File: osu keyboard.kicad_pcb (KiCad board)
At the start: 2 copper layers, 79.4 x 73.8 mm, 25 parts, among them SW1 SW_Push, U1 ATmega32U4-A, U2 PRTR5V0U2X, Y1 16MHz

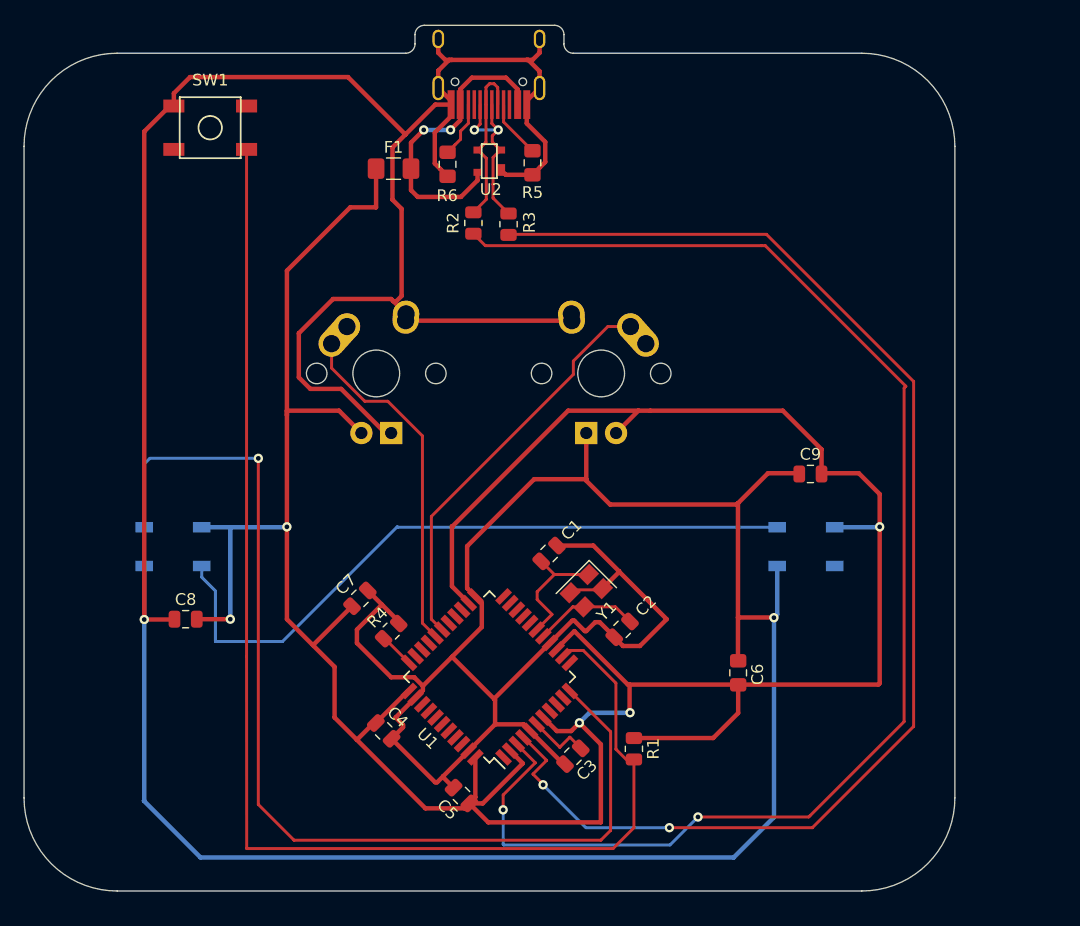
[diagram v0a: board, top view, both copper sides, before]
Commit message: using rp2040
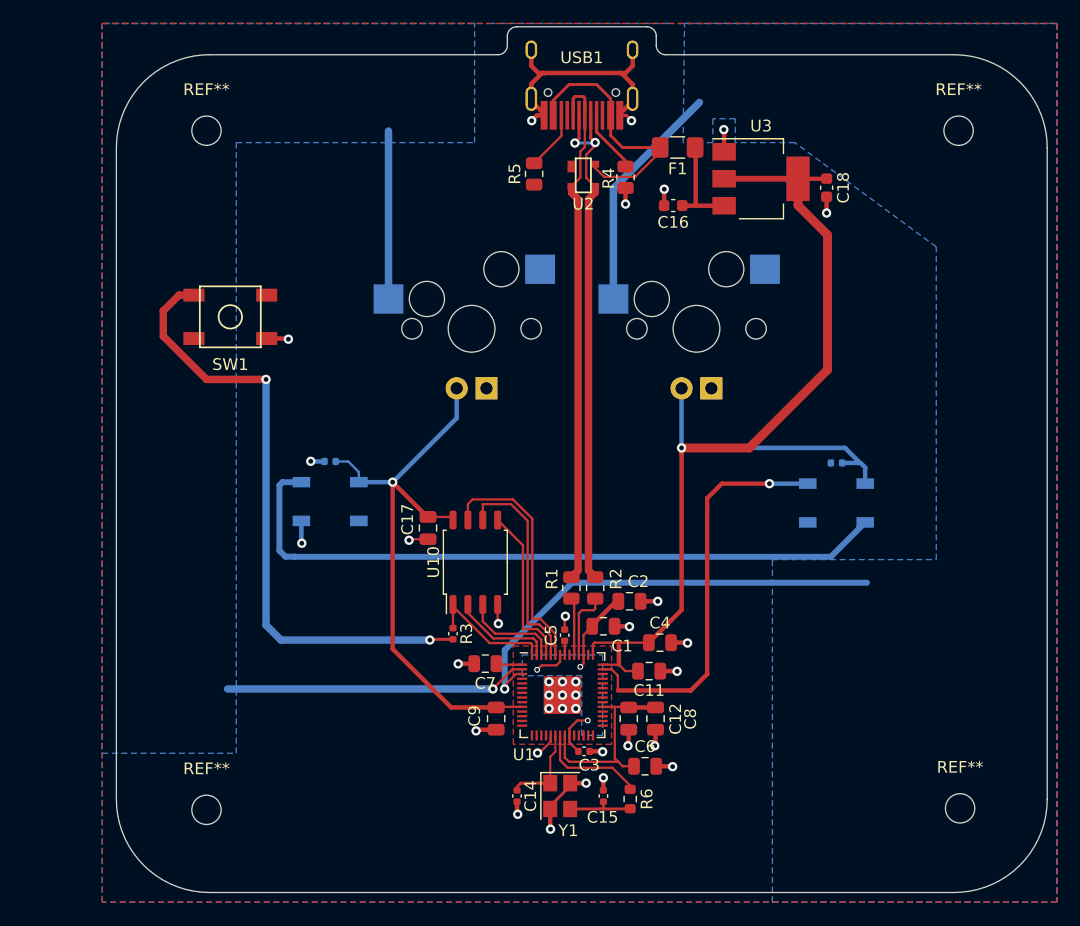
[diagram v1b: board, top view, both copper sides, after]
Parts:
- added C10: 100nF, Capacitor_SMD:C_0402_1005Metric, B.Cu at (156.6, 98.4)
- added C11: 100nF, Capacitor_SMD:C_0805_2012Metric, F.Cu at (140.6, 116.2)
- added C12: 100nF, Capacitor_SMD:C_0805_2012Metric, F.Cu at (138.9, 120.2)
- added C13: 100nF, Capacitor_SMD:C_0402_1005Metric, B.Cu at (113.4, 98.3)
- added C14: 14pF, Capacitor_SMD:C_0402_1005Metric, F.Cu at (129.3, 126.8)
- added C15: 14pF, Capacitor_SMD:C_0402_1005Metric, F.Cu at (136.7, 126.8)
- added C16: 22uF, Capacitor_SMD:C_0603_1608Metric, F.Cu at (142.7, 76.5)
- added C17: 100nF, Capacitor_SMD:C_0805_2012Metric, F.Cu at (121.8, 104.0)
- added C18: 22uF, Capacitor_SMD:C_0603_1608Metric, F.Cu at (155.7, 75.0)
- added REF**: MountingHole_2.5mm, MountingHole:MountingHole_2.5mm, F.Cu at (167.1, 127.9)
- added REF**: MountingHole_2.5mm, MountingHole:MountingHole_2.5mm, F.Cu at (167.0, 70.1)
- added REF**: MountingHole_2.5mm, MountingHole:MountingHole_2.5mm, F.Cu at (102.9, 70.1)
- added REF**: MountingHole_2.5mm, MountingHole:MountingHole_2.5mm, F.Cu at (102.9, 128.0)
- added U10: W25Q128JVS, Package_SO:SOIC-8_5.23x5.23mm_P1.27mm, F.Cu at (125.8, 106.9)
- added U3: AMS1117-3.3, Package_TO_SOT_SMD:SOT-223-3_TabPin2, F.Cu at (150.2, 74.2)
- C1, C2: value 22pF -> 100nF
- C3: footprint Capacitor_SMD:C_0805_2012Metric -> Capacitor_SMD:C_0402_1005Metric
- C4, C8, C9: value 0.1uF -> 100nF
- C5: value 0.1uF -> 1uF; footprint Capacitor_SMD:C_0805_2012Metric -> Capacitor_SMD:C_0402_1005Metric
- C6: value 10uF -> 100nF; footprint Capacitor_SMD:C_0805_2012Metric_Pad1.15x1.40mm_HandSolder -> Capacitor_SMD:C_0805_2012Metric
- C7: value 10uf -> 100nF
- F1: value 500mA -> Polyfuse_Small
- MX0: footprint MX_Alps_Hybrid:MX-1U -> MX_Only:MXOnly-1U-Hotswap-LED
- MX1: footprint MX_Alps_Hybrid:MX-1U -> MX_Only:MXOnly-1U-Hotswap-LED; moved to F.Cu
- R1: value 10k -> 27
- R2: value 22 -> 27
- R3: value 22 -> 1k; footprint Resistor_SMD:R_0805_2012Metric -> Capacitor_SMD:C_0402_1005Metric
- R4: value 10k -> 5.1k
- R5: footprint Resistor_SMD:R_0805_2012Metric_Pad1.15x1.40mm_HandSolder -> Resistor_SMD:R_0805_2012Metric
- R6: value 5.1k -> 1k; footprint Resistor_SMD:R_0805_2012Metric_Pad1.15x1.40mm_HandSolder -> Resistor_SMD:R_0603_1608Metric
- U1: value ATmega32U4-A -> RP2040; footprint Package_QFP:TQFP-44_10x10mm_P0.8mm -> Package_DFN_QFN:QFN-56-1EP_7x7mm_P0.4mm_EP3.2x3.2mm
- Y1: value 16MHz -> 12MHz
- moved D4 56.7 mm to (156.6, 101.9)
- moved R6 56.3 mm to (139.0, 127.1), turned to -90 degrees
- moved R4 43.6 mm to (138.6, 74.1), turned to 90 degrees
- moved C8 41.0 mm to (141.2, 120.2), turned to -90 degrees
- moved D1 40.8 mm to (113.4, 101.7)
- moved R3 35.2 mm to (123.9, 113.0)
- moved C9 34.0 mm to (127.6, 120.2), turned to -90 degrees
- moved R2 32.8 mm to (136.0, 109.1)
- moved C4 24.7 mm to (141.5, 113.8), turned to 0 degrees
- moved F1 24.3 mm to (143.0, 71.5), turned to 180 degrees
- moved Y1 17.7 mm to (133.0, 126.8), turned to -90 degrees
- moved C5 16.3 mm to (133.4, 113.1), turned to 90 degrees
- moved SW1 16.2 mm to (104.9, 86.0), turned to 0 degrees
- moved R1 14.7 mm to (134.0, 109.1)
- moved C7 12.1 mm to (126.6, 115.6), turned to 180 degrees
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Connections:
- net D- renamed /D-
- C1 pad 1: GND -> +1V1
- C1 pad 2: XTAL1 -> GND
- C2 pad 1: GND -> +1V1
- C2 pad 2: XTAL2 -> GND
- C3 pad 1: Net-(C3-Pad1) -> +1V1
- C4 pad 1: +5V -> +3V3
- C5 pad 1: +5V -> +3V3
- C6 pad 1: +5V -> +3V3
- C7 pad 1: +5V -> +3V3
- C8 pad 1: GND -> +3V3
- C8 pad 2: +5V -> GND
- C9 pad 1: GND -> +3V3
- C9 pad 2: +5V -> GND
- D1 pad 1: +5V -> +3V3
- D4 pad 1: +5V -> +3V3
- D4 pad 4: UNDERGLOWLED -> /UNDERGLOWLED
- F1 pad 1: +5V -> /REG
- MX0 pad 1: COL0 -> /COL0
- MX0 pad 3: +5V -> +3V3
- MX1 pad 1: COL1 -> /COL1
- MX1 pad 3: +5V -> +3V3
- R1 pad 1: +5V -> /D+
- R3 pad 1: D+ -> /QSPI_SS
- R4 pad 1: Net-(R4-Pad1) -> GND
- R4 pad 2: GND -> Net-(R4-Pad2)
- R5 pad 2: (no net) -> Net-(R5-Pad2)
- R6 pad 1: GND -> /XOUT
- R6 pad 2: (no net) -> Net-(C15-Pad1)
- SW1 pad 2: Net-(R1-Pad2) -> Net-(R3-Pad2)
- U1 pad 1: unconnected-(U1-Pad1) -> +3V3
- U1 pad 10: unconnected-(U1-Pad10) -> +3V3
- U1 pad 11: UNDERGLOWLED -> unconnected-(U1-Pad11)
- U1 pad 13: Net-(R1-Pad2) -> unconnected-(U1-Pad13)
- U1 pad 14: +5V -> unconnected-(U1-Pad14)
- U1 pad 15: GND -> unconnected-(U1-Pad15)
- U1 pad 16: XTAL2 -> unconnected-(U1-Pad16)
- U1 pad 17: XTAL1 -> unconnected-(U1-Pad17)
- U1 pad 19: unconnected-(U1-Pad19) -> GND
- U1 pad 2: +5V -> /COL0
- U1 pad 20: unconnected-(U1-Pad20) -> /XIN
- U1 pad 21: unconnected-(U1-Pad21) -> /XOUT
- U1 pad 22: unconnected-(U1-Pad22) -> +3V3
- U1 pad 23: GND -> +1V1
- U1 pad 24: +5V -> unconnected-(U1-Pad24)
- U1 pad 28: COL1 -> unconnected-(U1-Pad28)
- U1 pad 29: COL0 -> unconnected-(U1-Pad29)
- U1 pad 3: Net-(R2-Pad2) -> /COL1
- U1 pad 33: Net-(R4-Pad1) -> +3V3
- U1 pad 34: +5V -> unconnected-(U1-Pad34)
- U1 pad 35: GND -> unconnected-(U1-Pad35)
- U1 pad 4: Net-(R3-Pad2) -> unconnected-(U1-Pad4)
- U1 pad 41: unconnected-(U1-Pad41) -> /UNDERGLOWLED
- U1 pad 42: unconnected-(U1-Pad42) -> +3V3
- U1 pad 43: GND -> +3V3
- U1 pad 44: +5V -> +3V3
- U1 pad 5: GND -> unconnected-(U1-Pad5)
- U1 pad 6: Net-(C3-Pad1) -> unconnected-(U1-Pad6)
- U1 pad 7: +5V -> unconnected-(U1-Pad7)
- U2 pad 2: D+ -> /D+
- USB1 pad 10: (no net) -> Net-(R5-Pad2)
- USB1 pad 4: (no net) -> Net-(R4-Pad2)
- USB1 pad 6: D+ -> /D+
- USB1 pad 8: D+ -> /D+
- Y1 pad 1: XTAL1 -> /XIN
- Y1 pad 3: XTAL2 -> Net-(C15-Pad1)
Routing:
- net GND: track 422.7 -> 61.9 mm, vias 2 -> 36
- net +5V: track 264.8 -> 0.00 mm, vias 5 -> 0
- net +3V3: track 0.00 -> 165.0 mm, vias 0 -> 2
- net Net-(R2-Pad2): track 119.8 -> 5.97 mm, vias 2 -> 0
- net Net-(R1-Pad2): track 112.1 -> 4.89 mm
- net UNDERGLOWLED: track 89.8 -> 0.00 mm, vias 1 -> 0
- net /COL1: track 0.00 -> 58.6 mm, vias 0 -> 1
- net Net-(R3-Pad2): track 111.4 -> 53.1 mm
- net /D+: track 0.00 -> 44.4 mm
- net /COL0: track 0.00 -> 40.1 mm, vias 0 -> 1
- net /UNDERGLOWLED: track 0.00 -> 35.1 mm, vias 0 -> 1
- net COL1: track 34.4 -> 0.00 mm
- net /D-: track 14.5 -> 44.9 mm, vias 0 -> 2
- net COL0: track 29.8 -> 0.00 mm
- net /QSPI_SD3: track 0.00 -> 20.5 mm
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- added copper zone on B.Cu, net +1V1
- added copper zone on F.Cu, net +3V3
- added copper zone on B.Cu, net /COL0
- added copper zone on B.Cu, net /COL1
- added copper zone on B.Cu, net GND
- added copper zone on F.Cu, net GND
